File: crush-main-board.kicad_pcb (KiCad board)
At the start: 2 copper layers, 42 parts, among them J1 4x4_Header, J10 3x3 Header, J11 3x3 Header, J12 3x2 Header, J13 3x4_Header, J14 3x4_Header, J15 2157601008, J16 Conn_01x02, J17 Conn_01x02, J2 4x4_Header, J3 6x2_Header, J4 3x1_Header, J5 3x2 Header, J6 3x2 Header, J7 3x4 Header, J8 3x4 Header, J9 3x3 Header, Q1 BSN20, Q2 BSN20, Q3 BSN20, Q5 DMG2301L, U1 Teensy4.1, U2 ISO7740DW, U3 ISO7740DW, U4 ISO1640BDR, U5 INA232B, U6 INA232B

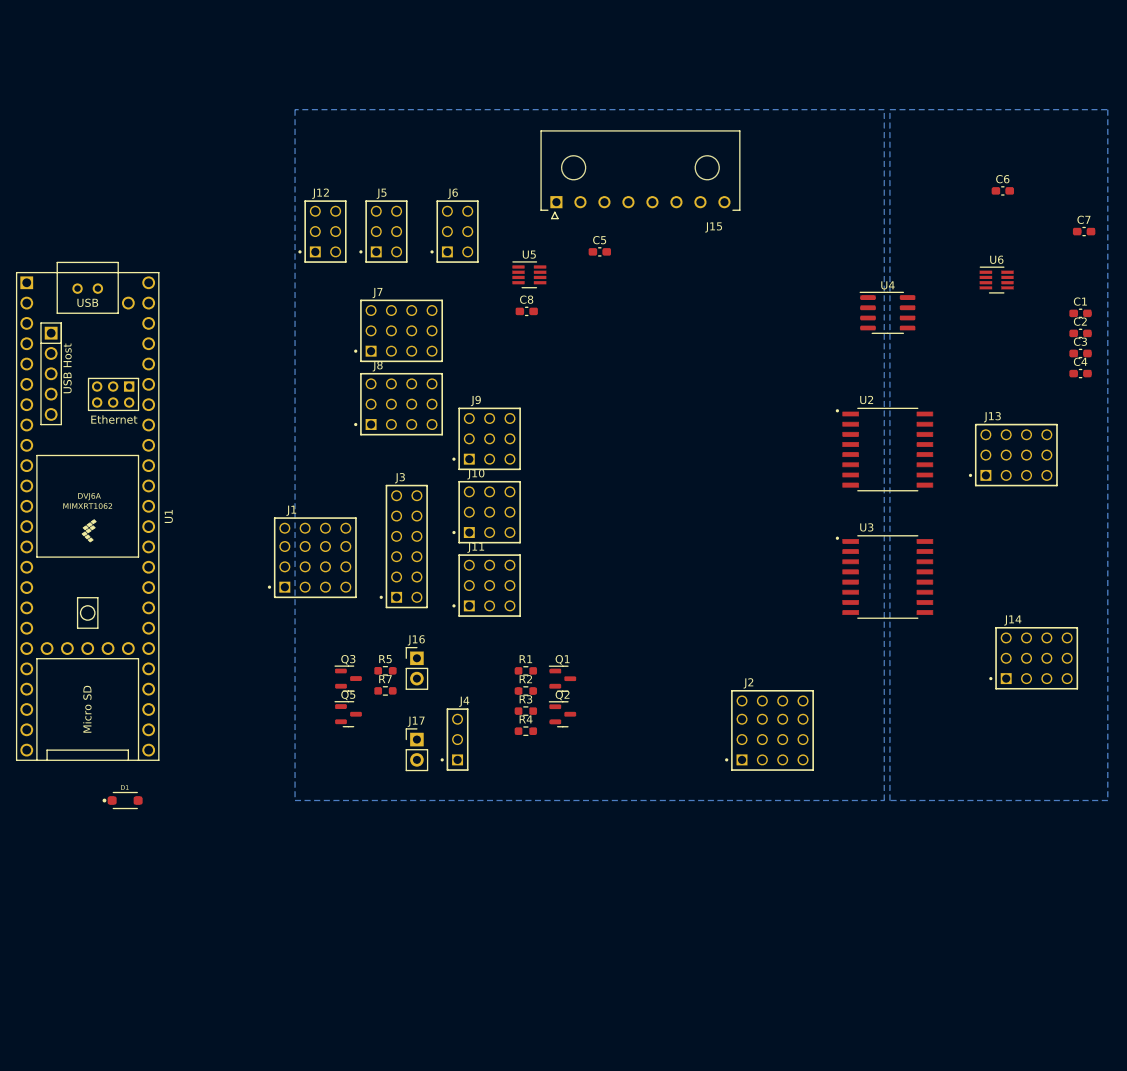
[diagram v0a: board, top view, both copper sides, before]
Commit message: basic routing
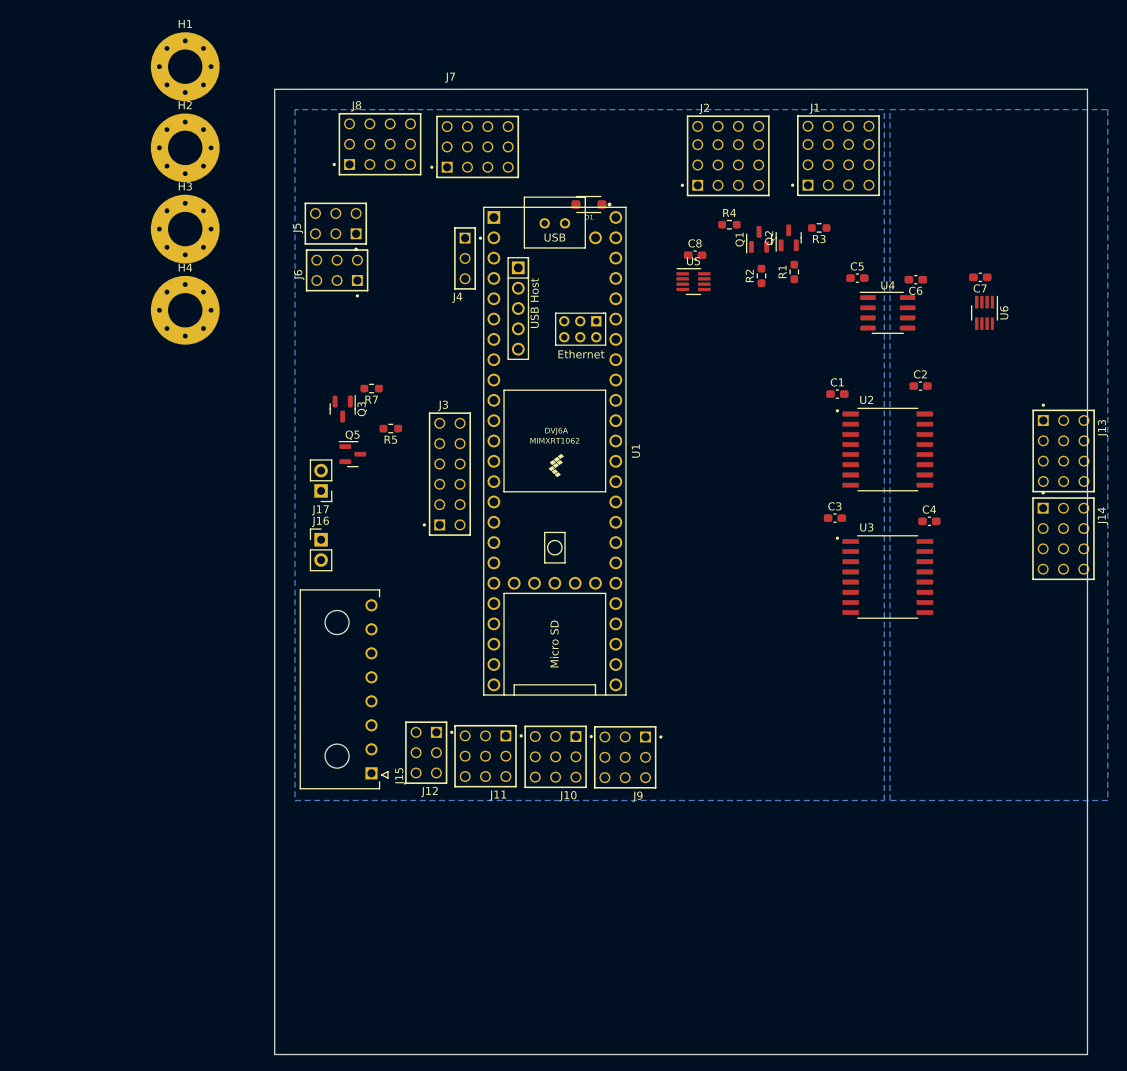
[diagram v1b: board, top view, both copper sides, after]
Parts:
- added H1: MountingHole_Pad, MountingHole:MountingHole_4.3mm_M4_Pad_Via, F.Cu at (1.52, 9.87)
- added H2: MountingHole_Pad, MountingHole:MountingHole_4.3mm_M4_Pad_Via, F.Cu at (1.52, 20.0)
- added H3: MountingHole_Pad, MountingHole:MountingHole_4.3mm_M4_Pad_Via, F.Cu at (1.52, 30.2)
- added H4: MountingHole_Pad, MountingHole:MountingHole_4.3mm_M4_Pad_Via, F.Cu at (1.52, 40.3)
- moved D1 94.4 mm to (52.0, 27.1), turned to 180 degrees
- moved J1 82.5 mm to (83.2, 20.9)
- moved J15 75.0 mm to (24.8, 98.2), turned to -90 degrees
- moved J2 72.0 mm to (69.4, 20.9)
- moved R3 70.7 mm to (80.8, 30.0), turned to 180 degrees
- moved R4 68.2 mm to (69.5, 29.6)
- moved J12 66.4 mm to (31.6, 95.6), turned to 180 degrees
- moved Q2 65.9 mm to (77.0, 31.3), turned to 90 degrees
- moved J4 60.1 mm to (36.5, 33.8), turned to 180 degrees
- moved Q1 60.1 mm to (73.2, 31.5), turned to 90 degrees
- moved R1 60.1 mm to (77.7, 35.5), turned to 90 degrees
- moved R2 59.7 mm to (73.5, 36.0), turned to 90 degrees
- moved U1 59.0 mm to (47.7, 57.9)
- moved J9 43.3 mm to (56.5, 96.2), turned to 180 degrees
- moved R7 37.8 mm to (24.8, 50.1), turned to 180 degrees
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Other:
- board outline added: 101.6 x 120.6 mm
